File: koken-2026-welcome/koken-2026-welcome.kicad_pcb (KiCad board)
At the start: 2 copper layers, 44 x 44 mm, 22 parts, among them J1 USB_C_Receptacle_USB2.0_16P, J2 Conn_01x03_Pin, SW1 SW_Push, SW2 SW_SPDT, U1 CH32V003JxMx, U2 AP7333

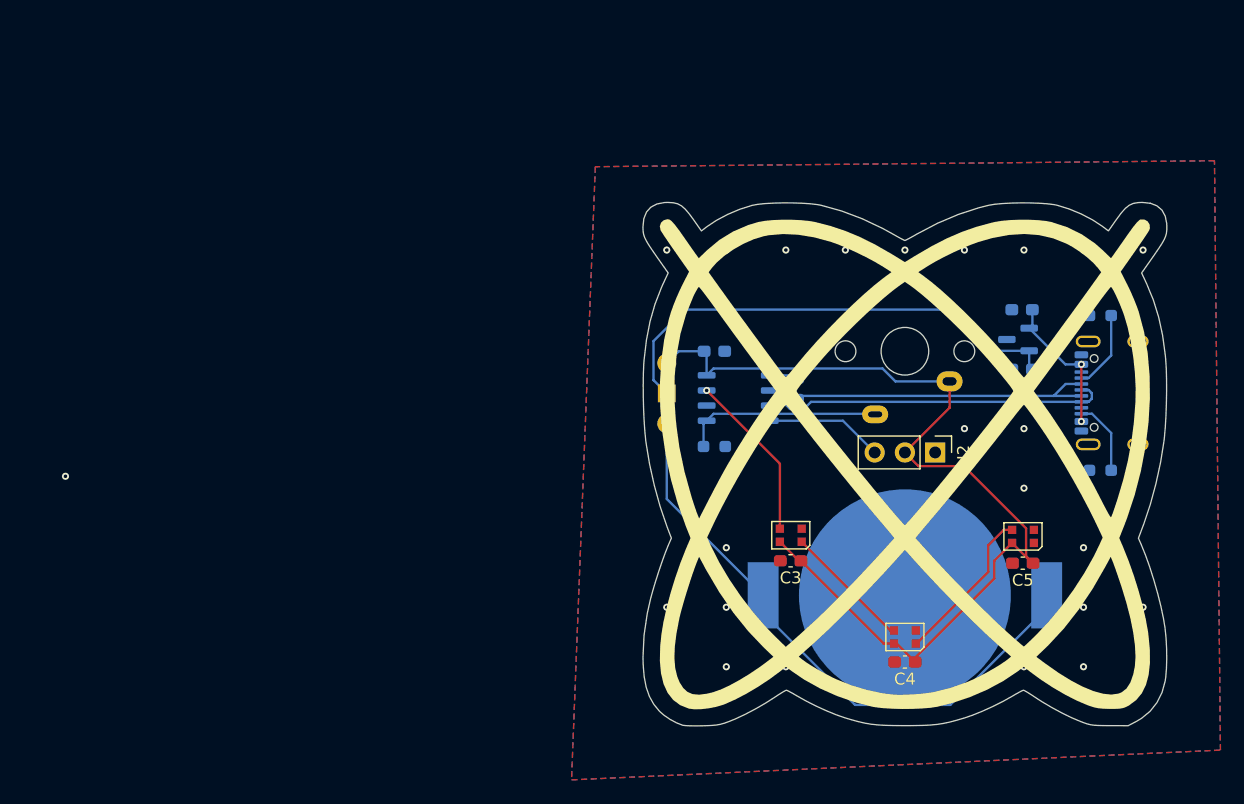
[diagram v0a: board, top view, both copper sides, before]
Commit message: pro
Co-authored-by: Mcbeeringi⁉️ <git@mcbeeringi.dev>
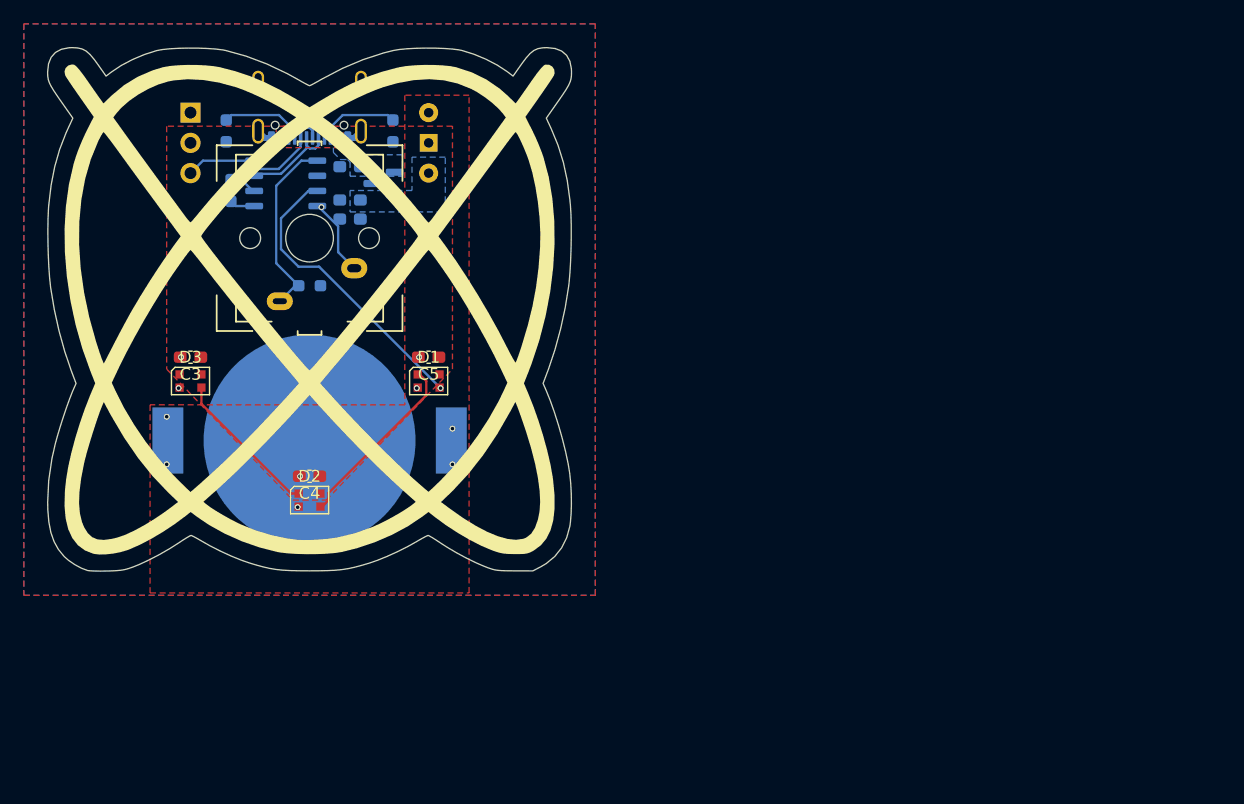
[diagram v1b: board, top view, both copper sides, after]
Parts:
- J2: moved to B.Cu
- moved R1 75.0 mm to (93.0, 85.0), turned to -90 degrees
- moved J1 73.0 mm to (100.0, 81.9), turned to 0 degrees
- moved D3 71.1 mm to (90.0, 106.0), turned to 0 degrees
- moved J2 68.7 mm to (90.0, 83.5), turned to 180 degrees
- moved R2 65.9 mm to (107.0, 85.0), turned to -90 degrees
- moved C2 58.2 mm to (103.4, 90.8)
- moved C1 57.7 mm to (103.4, 88.0)
- moved U2 54.9 mm to (106.1, 87.9)
- moved C3 53.2 mm to (90.0, 104.0)
- moved C5 52.8 mm to (110.0, 104.0)
- moved C4 52.4 mm to (100.0, 114.0)
- moved BT1 51.7 mm to (100.0, 111.0)
- moved G*** 51.7 mm to (100.0, 100.0) (x2)
- moved D2 51.3 mm to (100.0, 116.0), turned to 0 degrees
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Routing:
- net VDD: track 81.6 -> 6.54 mm, vias 0 -> 1
- net BAT: track 50.7 -> 0.00 mm, vias 0 -> 4
- net +3.3V: track 40.6 -> 0.00 mm
- net D+: track 28.9 -> 8.66 mm
- net D-: track 29.4 -> 12.1 mm
- net +5V: track 12.1 -> 0.00 mm, vias 2 -> 4
- net WS2812C: track 14.2 -> 24.8 mm
- net Net-(D1-DOUT): track 10.8 -> 15.3 mm
- net SWIO: track 9.91 -> 5.78 mm
- net GND: track 0.00 -> 2.72 mm, vias 25 -> 6
- net KEY: track 16.7 -> 15.6 mm
- net Net-(D2-DOUT): track 13.3 -> 12.7 mm
- net (no net): vias 2 -> 0
- added copper zone on B.Cu, net +3.3V
- added copper zone on B.Cu, net +5V
- added copper zone on F.Cu, net +5V
- added copper zone on F.Cu, net BAT
- added copper zone on F.Cu, net VDD
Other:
- outline, holes or cut-outs redrawn
